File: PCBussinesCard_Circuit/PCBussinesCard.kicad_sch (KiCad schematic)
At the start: 17 parts, among them IC1 NT2H1311F0DTL, J1 Conn_ARM_JTAG_SWD_10, J2 USB_A_PCB, J3 Conn_01x13_Pin, J4 Conn_01x13_Pin, U1 STM32L552CCTx, U2 AP7370-33FDC

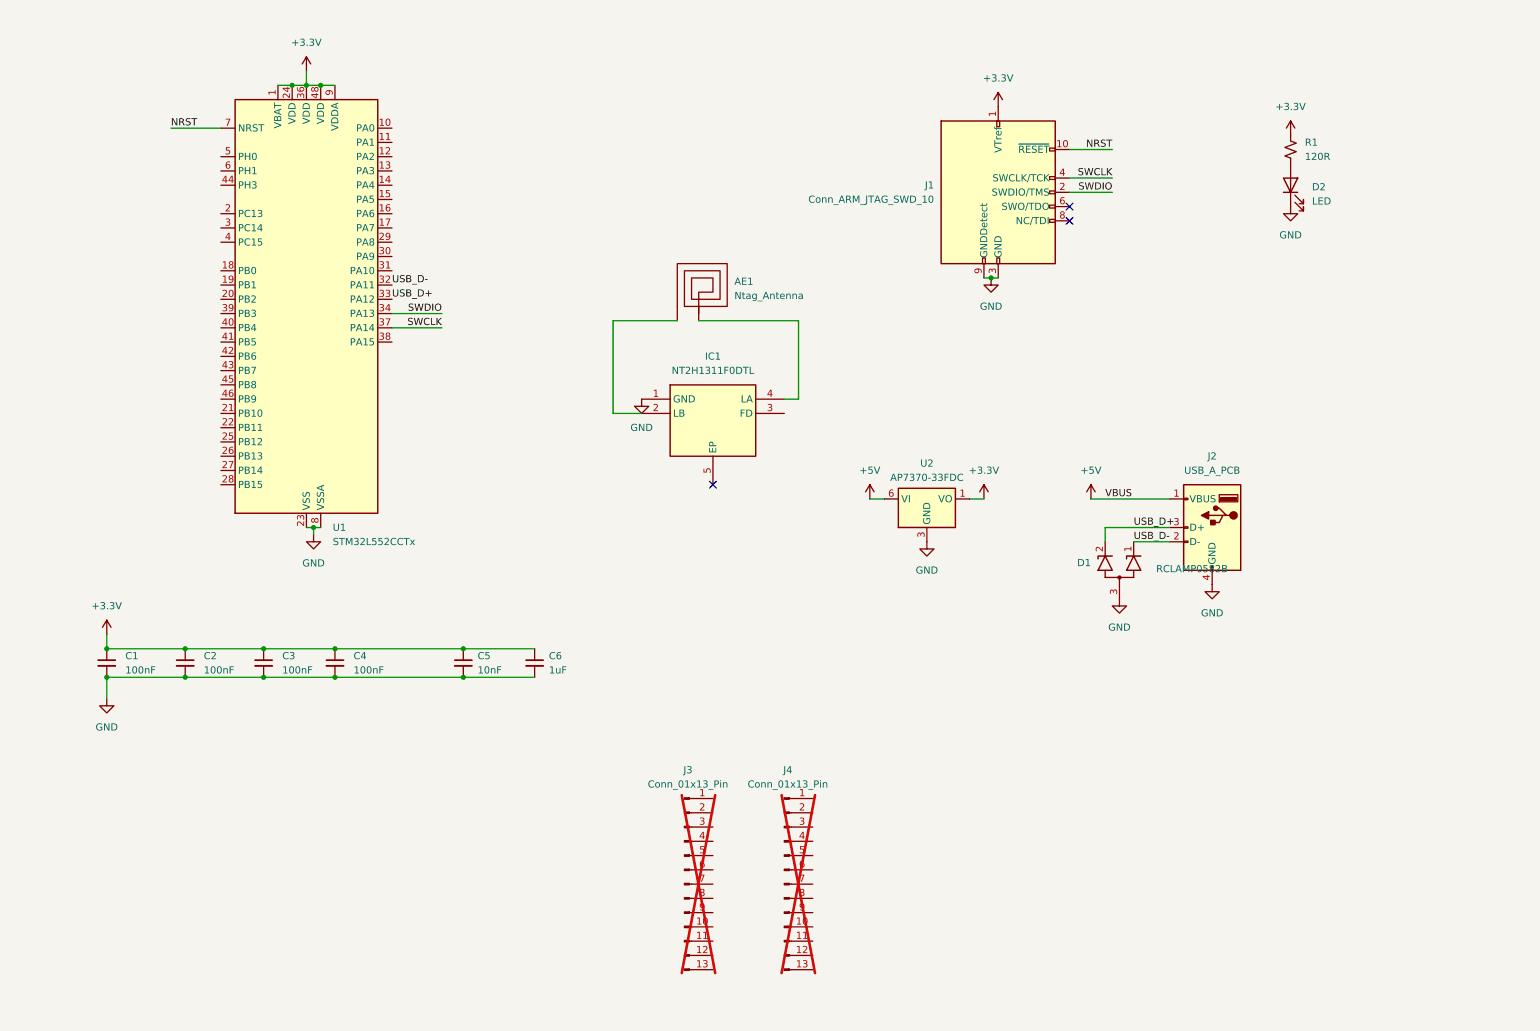
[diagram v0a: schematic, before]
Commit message: cleanup and reorganizing
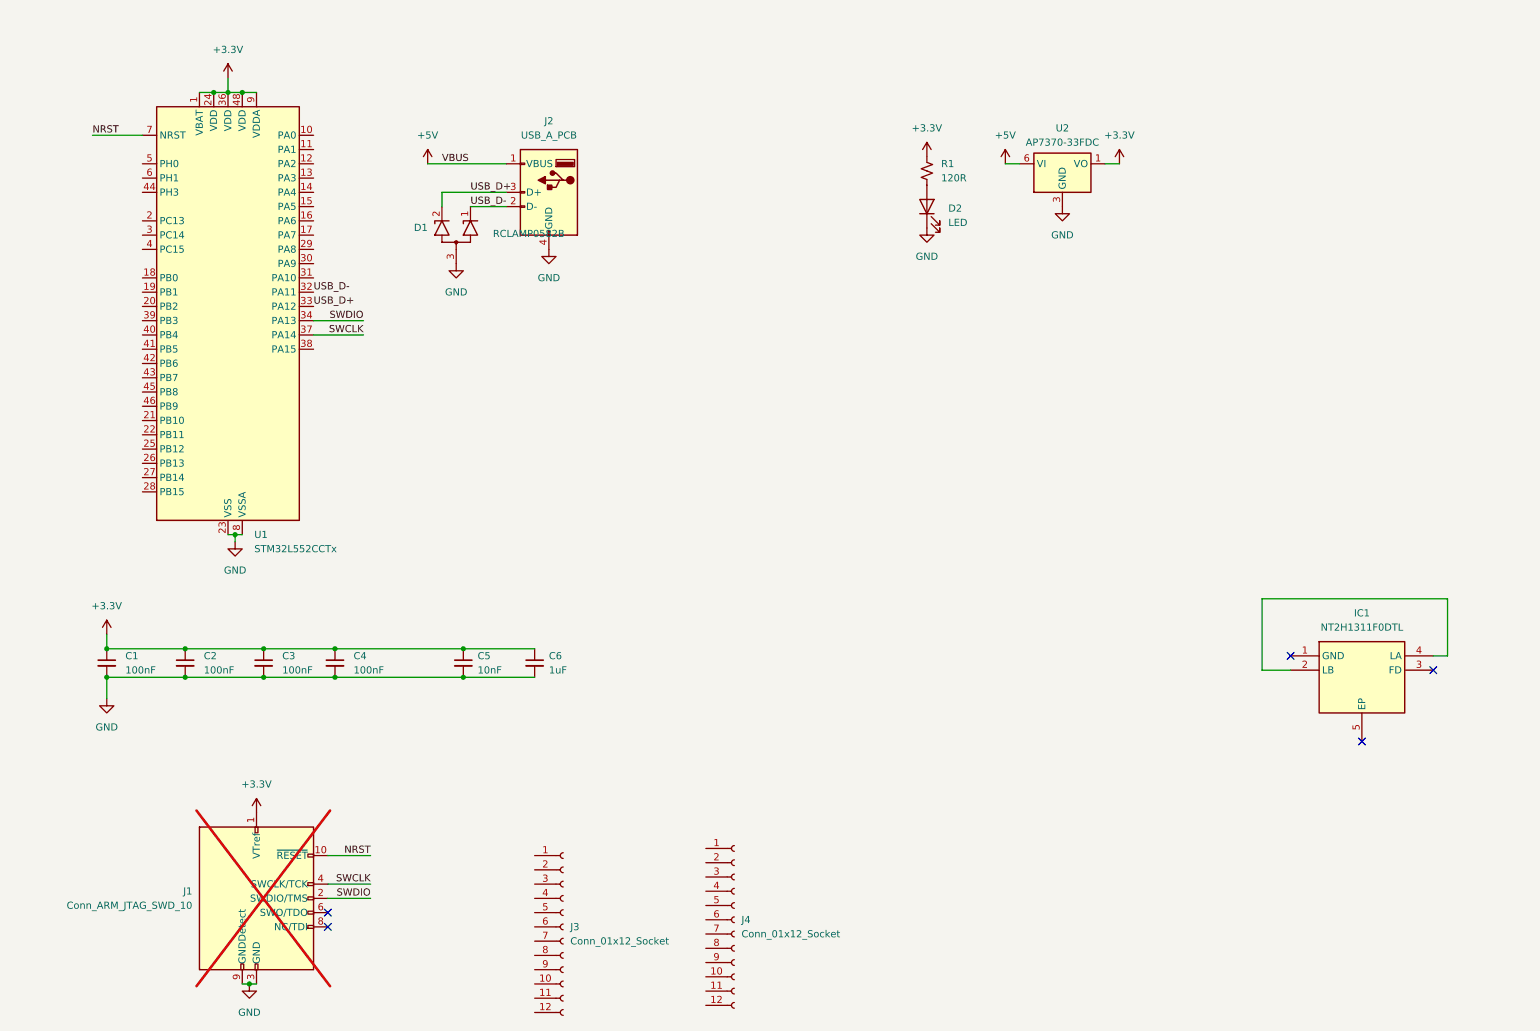
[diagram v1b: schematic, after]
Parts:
- removed AE1: Ntag_Antenna, ProjectLibrary:Ntag_Antenna, symbol Project_library:Ntag_Antenna
- removed J3, J4: Conn_01x13_Pin, Connector_PinHeader_2.54mm:PinHeader_1x13_P2.54mm_Vertical, symbol Connector:Conn_01x13_Pin
- added J3, J4: Conn_01x12_Socket, Connector_PinHeader_2.54mm:PinHeader_1x12_P2.54mm_Vertical, symbol Connector:Conn_01x12_Socket
- J1: now not fitted
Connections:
- net GND: no longer IC1.1 (GND)
- net at IC1.2 (LB): now also IC1.4 (LA)
- no-connect marks 3 -> 5
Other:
- moved on the sheet: D1, D2, IC1, J2, R1, U1, U2

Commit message: Version 1.0
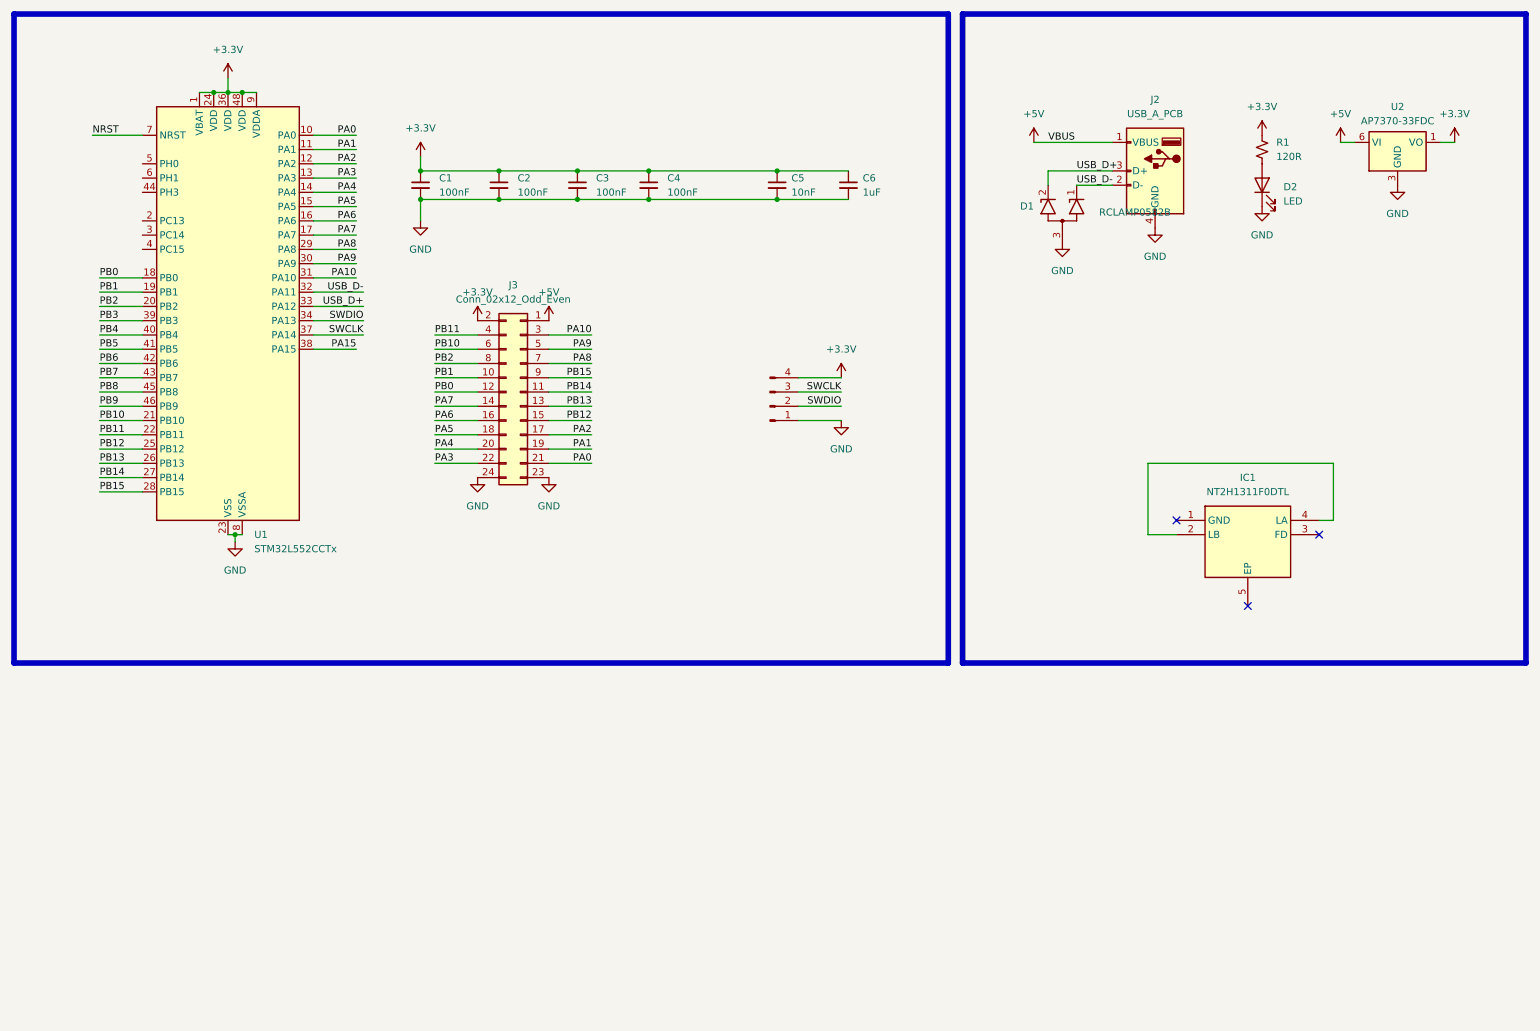
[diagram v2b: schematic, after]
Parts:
- removed J1: Conn_ARM_JTAG_SWD_10, Connector_PinHeader_1.27mm:PinHeader_2x05_P1.27mm_Vertical_SMD, symbol Connector:Conn_ARM_JTAG_SWD_10
- removed J3, J4: Conn_01x12_Socket, Connector_PinHeader_2.54mm:PinHeader_1x12_P2.54mm_Vertical, symbol Connector:Conn_01x12_Socket
- added J1: Conn_01x04_Pin, Connector_PinHeader_2.54mm:PinHeader_1x04_P2.54mm_Horizontal, symbol Connector:Conn_01x04_Pin
- added J3: Conn_02x12_Odd_Even, Connector_PinSocket_2.54mm:PinSocket_2x12_P2.54mm_Vertical, symbol Connector_Generic:Conn_02x12_Odd_Even
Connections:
- net +3.3V: now also J1.4 (Pin_4), J3.2 (Pin_2)
- net +5V: now also J3.1 (Pin_1)
- net GND: now also J1.1 (Pin_1), J3.23 (Pin_23), J3.24 (Pin_24)
- net SWCLK: now also J1.3 (Pin_3)
- net SWDIO: now also J1.2 (Pin_2)
- net PA0: now reaches U1.10 (PA0)
- net PA0: now also J3.21 (Pin_21)
- net PA1: now reaches U1.11 (PA1)
- net PA1: now also J3.19 (Pin_19)
- net PA2: now reaches U1.12 (PA2)
- net PA2: now also J3.17 (Pin_17)
- net PA3: now reaches U1.13 (PA3)
- net PA3: now also J3.22 (Pin_22)
- net PA4: now reaches U1.14 (PA4)
- net PA4: now also J3.20 (Pin_20)
- net PA5: now reaches U1.15 (PA5)
- net PA5: now also J3.18 (Pin_18)
- net PA6: now reaches U1.16 (PA6)
- net PA6: now also J3.16 (Pin_16)
- net PA7: now reaches U1.17 (PA7)
- net PA7: now also J3.14 (Pin_14)
- net PB0: now reaches U1.18 (PB0)
- net PB0: now also J3.12 (Pin_12)
- net PB1: now reaches U1.19 (PB1)
- net PB1: now also J3.10 (Pin_10)
- net PB2: now reaches U1.20 (PB2)
- net PB2: now also J3.8 (Pin_8)
- net PB10: now reaches U1.21 (PB10)
- net PB10: now also J3.6 (Pin_6)
- net PB11: now reaches U1.22 (PB11)
- net PB11: now also J3.4 (Pin_4)
- net PB12: now reaches U1.25 (PB12)
- net PB12: now also J3.15 (Pin_15)
- net PB13: now reaches U1.26 (PB13)
- net PB13: now also J3.13 (Pin_13)
- net PB14: now reaches U1.27 (PB14)
- net PB14: now also J3.11 (Pin_11)
- net PB15: now reaches U1.28 (PB15)
- net PB15: now also J3.9 (Pin_9)
- net PA8: now reaches U1.29 (PA8)
- net PA8: now also J3.7 (Pin_7)
- net PA9: now reaches U1.30 (PA9)
- net PA9: now also J3.5 (Pin_5)
- net PA10: now reaches U1.31 (PA10)
- net PA10: now also J3.3 (Pin_3)
- net PA15: now reaches U1.38 (PA15)
- net PB3: now reaches U1.39 (PB3)
- net PB4: now reaches U1.40 (PB4)
- net PB5: now reaches U1.41 (PB5)
- net PB6: now reaches U1.42 (PB6)
- net PB7: now reaches U1.43 (PB7)
- net PB8: now reaches U1.45 (PB8)
- net PB9: now reaches U1.46 (PB9)
- no-connect marks 5 -> 3
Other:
- moved on the sheet: C1, C2, C3, C4, C5, C6, D1, D2, IC1, J2, R1, U2

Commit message: Production V1.0
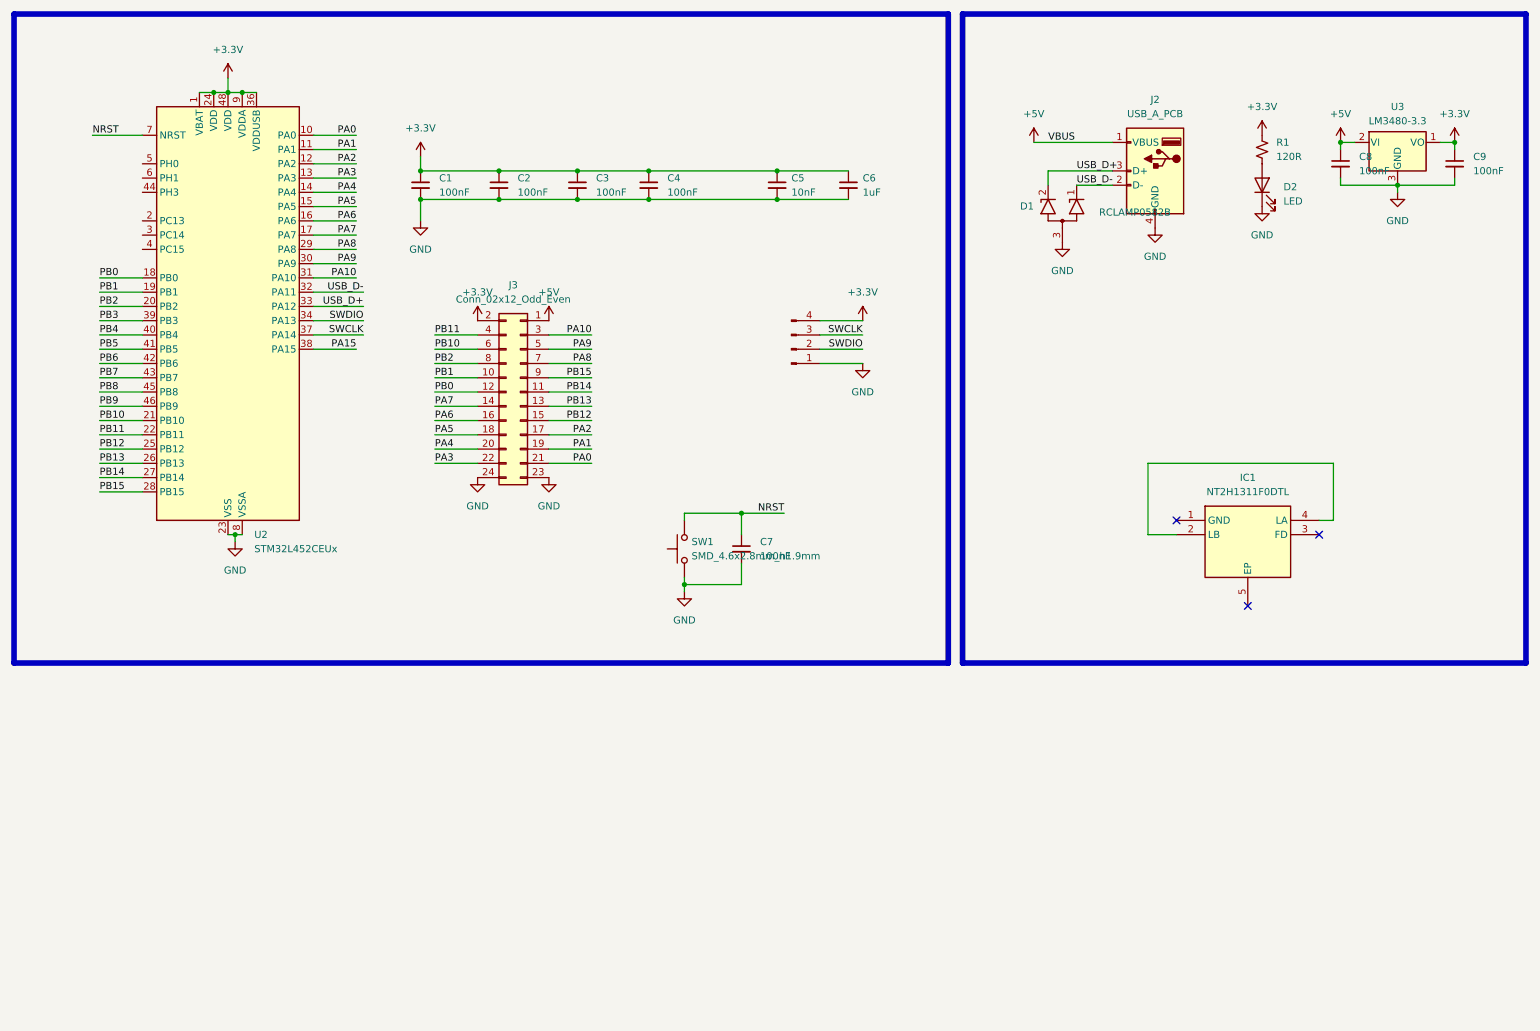
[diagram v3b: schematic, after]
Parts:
- removed U1: STM32L552CCTx, Package_QFP:LQFP-48_7x7mm_P0.5mm, symbol MCU_ST_STM32L5:STM32L552CCTx
- removed U2: AP7370-33FDC, Package_DFN_QFN:DFN-6-1EP_2x2mm_P0.65mm_EP1.01x1.7mm, symbol Regulator_Linear:AP7370-33FDC
- added C7, C8, C9: 100nF, Capacitor_SMD:C_0402_1005Metric, symbol Device:C_Small
- added SW1: SMD_4.6x2.8mm_h1.9mm, PCM_SparkFun-Switch:Push_SMD_4.6x2.8mm_h1.9mm, symbol PCM_SparkFun-Switch:SPST_Push_SMD_4.6x2.8mm_h1.9mm
- added U2: STM32L452CEUx, Package_DFN_QFN:QFN-48-1EP_7x7mm_P0.5mm_EP5.6x5.6mm, symbol MCU_ST_STM32L4:STM32L452CEUx
- added U3: LM3480-3.3, Package_TO_SOT_SMD:SOT-23, symbol Regulator_Linear:LM3480-3.3
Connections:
- net +3.3V: now also C9.1, U2.1 (VBAT), U2.24 (VDD), U2.36 (VDDUSB), U2.48 (VDD), U2.9 (VDDA), U3.1 (VO)
- net +5V: now also C8.1, U3.2 (VI)
- net GND: now also C7.2, C8.2, C9.2, SW1.1, U2.23 (VSS), U2.35 (VSS), U2.47 (VSS), U2.49 (VSS), U2.8 (VSSA), U3.3 (GND)
- net NRST: now also C7.1, SW1.2, U2.7 (NRST)
- net PA0: now also U2.10 (PA0)
- net PA1: now also U2.11 (PA1)
- net PA10: now also U2.31 (PA10)
- net PA15: now also U2.38 (PA15)
- net PA2: now also U2.12 (PA2)
- net PA3: now also U2.13 (PA3)
- net PA4: now also U2.14 (PA4)
- net PA5: now also U2.15 (PA5)
- net PA6: now also U2.16 (PA6)
- net PA7: now also U2.17 (PA7)
- net PA8: now also U2.29 (PA8)
- net PA9: now also U2.30 (PA9)
- net PB0: now also U2.18 (PB0)
- net PB1: now also U2.19 (PB1)
- net PB10: now also U2.21 (PB10)
- net PB11: now also U2.22 (PB11)
- net PB12: now also U2.25 (PB12)
- net PB13: now also U2.26 (PB13)
- net PB14: now also U2.27 (PB14)
- net PB15: now also U2.28 (PB15)
- net PB2: now also U2.20 (PB2)
- net PB3: now also U2.39 (PB3)
- net PB4: now also U2.40 (PB4)
- net PB5: now also U2.41 (PB5)
- net PB6: now also U2.42 (PB6)
- net PB7: now also U2.43 (PB7)
- net PB8: now also U2.45 (PB8)
- net PB9: now also U2.46 (PB9)
- net SWCLK: now also U2.37 (PA14)
- net SWDIO: now also U2.34 (PA13)
- net USB_D+: now also U2.33 (PA12)
- net USB_D-: now also U2.32 (PA11)
